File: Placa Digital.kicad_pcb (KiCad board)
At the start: 2 copper layers, 60 x 80 mm, 23 parts, among them J1 Entradas / Salidas, Q1 BC548, Q2 BC548, U1 EC11_Module, U2 Alimentación, U3 ST7920_Display, U4 10K

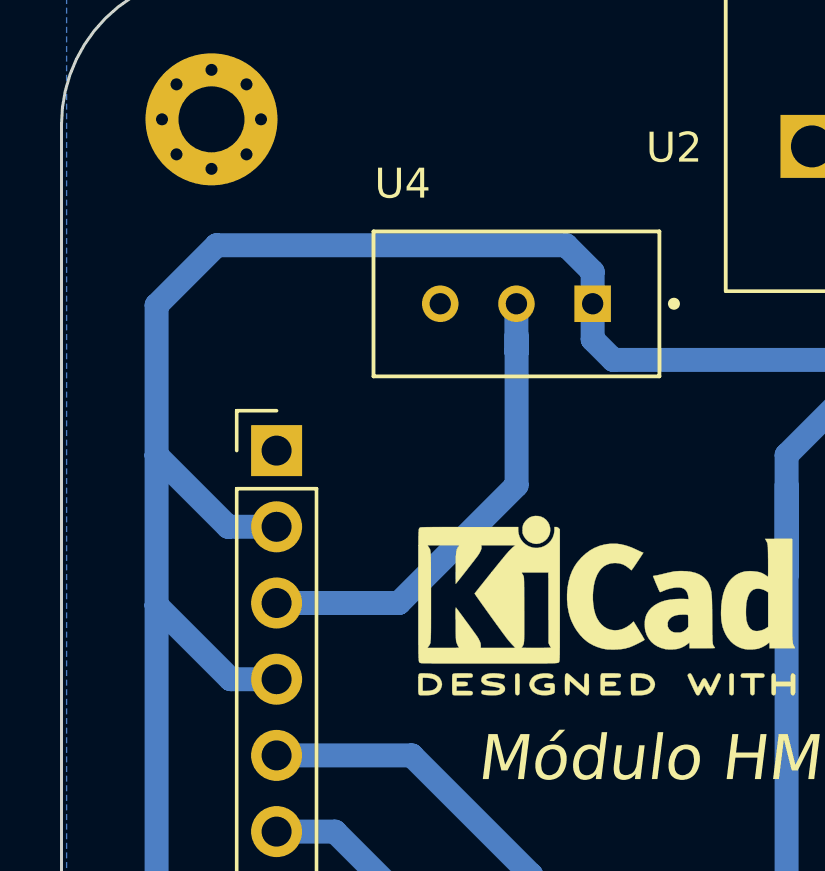
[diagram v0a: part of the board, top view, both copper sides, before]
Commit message: Layout modified + Gerbers generated
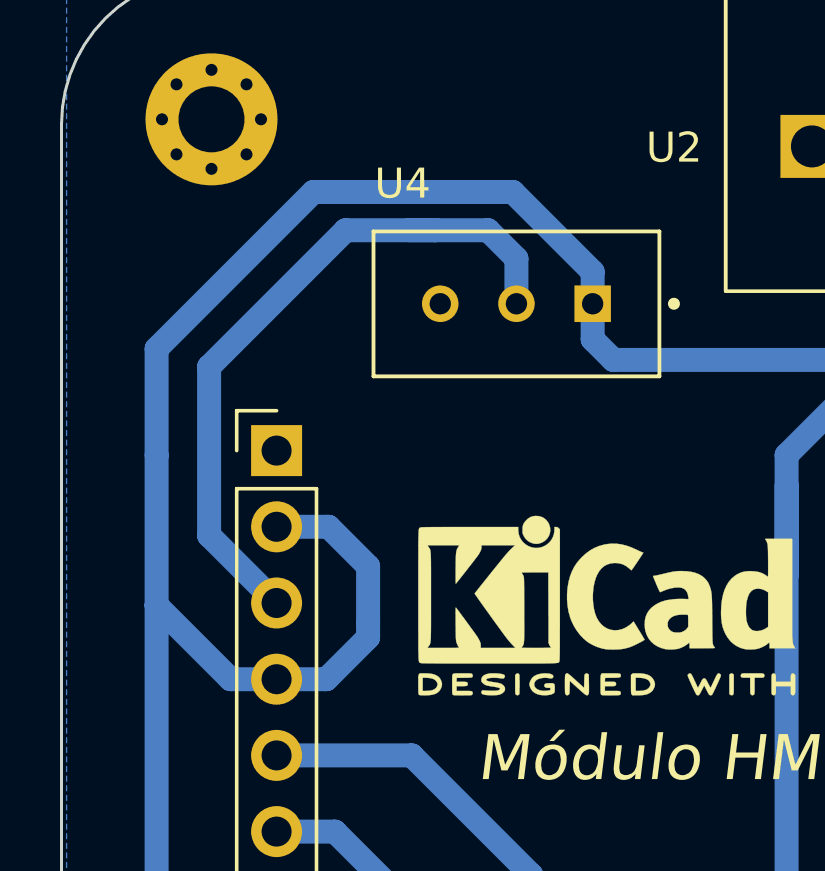
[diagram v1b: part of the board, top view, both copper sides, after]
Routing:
- net Net-(U3-Pad3): track 16.2 -> 23.7 mm
- net +5V: track 123.2 -> 128.5 mm
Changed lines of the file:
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@@
   (segment (start 143.61879 105.35221) (end 143.652 105.319) (width 0.8) (layer "B.Cu") (net 23))
   (segment (start 137.6645 105.35221) (end 143.61879 105.35221) (width 0.8) (layer "B.Cu") (net 23))
-  (segment (start 125.612 71.864) (end 125.617 71.869) (width 0.8) (layer "B.Cu") (net 24))
-  (segment (start 125.612 70.269) (end 125.612 71.864) (width 0.8) (layer "B.Cu") (net 24))
-  (segment (start 121.692 80.244) (end 125.617 76.319) (width 0.8) (layer "B.Cu") (net 24))
-  (segment (start 125.617 71.869) (end 125.617 71.319) (width 0.8) (layer "B.Cu") (net 24))
-  (segment (start 125.617 76.319) (end 125.617 71.869) (width 0.8) (layer "B.Cu") (net 24))
-  (segment (start 117.617 80.244) (end 121.692 80.244) (width 0.8) (layer "B.Cu") (net 24))
+  (segment (start 115.367 72.369) (end 119.917 67.819) (width 0.8) (layer "B.Cu") (net 24))
+  (segment (start 115.367 77.994) (end 115.367 72.369) (width 0.8) (layer "B.Cu") (net 24))
+  (segment (start 125.612 68.764) (end 124.667 67.819) (width 0.8) (layer "B.Cu") (net 24))
+  (segment (start 117.617 80.244) (end 115.367 77.994) (width 0.8) (layer "B.Cu") (net 24))
+  (segment (start 122.917 67.819) (end 122.017 67.819) (width 0.8) (layer "B.Cu") (net 24))
+  (segment (start 119.917 67.819) (end 122.917 67.819) (width 0.8) (layer "B.Cu") (net 24))
+  (segment (start 125.612 70.269) (end 125.612 68.764) (width 0.8) (layer "B.Cu") (net 24))
+  (segment (start 124.667 67.819) (end 122.917 67.819) (width 0.8) (layer "B.Cu") (net 24))
+  (segment (start 128.152 69.204) (end 125.492 66.544) (width 0.8) (layer "B.Cu") (net 26))
+  (segment (start 120.667 81.394) (end 120.667 80.919) (width 0.8) (layer "B.Cu") (net 26))
   (segment (start 128.8395 72.1415) (end 137.7895 72.1415) (width 0.8) (layer "B.Cu") (net 26))
   (segment (start 140.462 65.024) (end 140.462 69.469) (width 0.8) (layer "B.Cu") (net 26))
+  (segment (start 120.667 79.019) (end 120.667 80.919) (width 0.8) (layer "B.Cu") (net 26))
   (segment (start 113.617 80.319) (end 113.617 75.319) (width 0.8) (layer "B.Cu") (net 26))
   (segment (start 140.462 69.469) (end 139.6145 70.3165) (width 0.8) (layer "B.Cu") (net 26))
-  (segment (start 127.267 68.319) (end 115.617 68.319) (width 0.8) (layer "B.Cu") (net 26))
-  (segment (start 117.617 77.704) (end 116.002 77.704) (width 0.8) (layer "B.Cu") (net 26))
+  (segment (start 125.492 66.544) (end 118.842 66.544) (width 0.8) (layer "B.Cu") (net 26))
   (segment (start 137.037 92.329) (end 137.037 96.774) (width 0.8) (layer "B.Cu") (net 26))
-  (segment (start 115.617 68.319) (end 113.617 70.319) (width 0.8) (layer "B.Cu") (net 26))
   (segment (start 117.617 115.804) (end 113.617 111.804) (width 0.8) (layer "B.Cu") (net 26))
   (segment (start 128.152 71.454) (end 128.8395 72.1415) (width 0.8) (layer "B.Cu") (net 26))
-  (segment (start 128.152 70.269) (end 128.152 69.204) (width 0.8) (layer "B.Cu") (net 26))
+  (segment (start 118.842 66.544) (end 113.617 71.769) (width 0.8) (layer "B.Cu") (net 26))
   (segment (start 134.617 89.909) (end 134.617 75.314) (width 0.8) (layer "B.Cu") (net 26))
-  (segment (start 128.152 69.204) (end 127.267 68.319) (width 0.8) (layer "B.Cu") (net 26))
+  (segment (start 117.617 77.704) (end 119.352 77.704) (width 0.8) (layer "B.Cu") (net 26))
   (segment (start 134.617 75.314) (end 137.7895 72.1415) (width 0.8) (layer "B.Cu") (net 26))
+  (segment (start 113.617 71.769) (end 113.617 75.319) (width 0.8) (layer "B.Cu") (net 26))
   (segment (start 117.617 82.784) (end 116.082 82.784) (width 0.8) (layer "B.Cu") (net 26))
   (segment (start 137.037 92.329) (end 134.617 89.909) (width 0.8) (layer "B.Cu") (net 26))
+  (segment (start 119.277 82.784) (end 120.667 81.394) (width 0.8) (layer "B.Cu") (net 26))
+  (segment (start 119.352 77.704) (end 120.667 79.019) (width 0.8) (layer "B.Cu") (net 26))
   (segment (start 134.617 79.319) (end 134.617 76.319) (width 0.8) (layer "B.Cu") (net 26))
   (segment (start 128.152 70.269) (end 128.152 71.454) (width 0.8) (layer "B.Cu") (net 26))
   (segment (start 116.082 82.784) (end 113.617 80.319) (width 0.8) (layer "B.Cu") (net 26))
-  (segment (start 116.002 77.704) (end 113.617 75.319) (width 0.8) (layer "B.Cu") (net 26))
+  (segment (start 117.617 82.784) (end 119.277 82.784) (width 0.8) (layer "B.Cu") (net 26))
   (segment (start 113.617 111.804) (end 113.617 80.319) (width 0.8) (layer "B.Cu") (net 26))
   (segment (start 137.7895 72.1415) (end 139.6145 70.3165) (width 0.8) (layer "B.Cu") (net 26))
-  (segment (start 113.617 70.319) (end 113.617 75.319) (width 0.8) (layer "B.Cu") (net 26))
+  (segment (start 128.152 70.269) (end 128.152 69.204) (width 0.8) (layer "B.Cu") (net 26))
   (zone (net 25) (net_name "GND") (layer "B.Cu") (hatch edge 0.508)
     (connect_pads (clearance 0.508))
